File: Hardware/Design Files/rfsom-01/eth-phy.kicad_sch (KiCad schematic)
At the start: 50 parts, among them U6 KSZ9131RNXI-TR, Y3 ECS-2033-250-BN

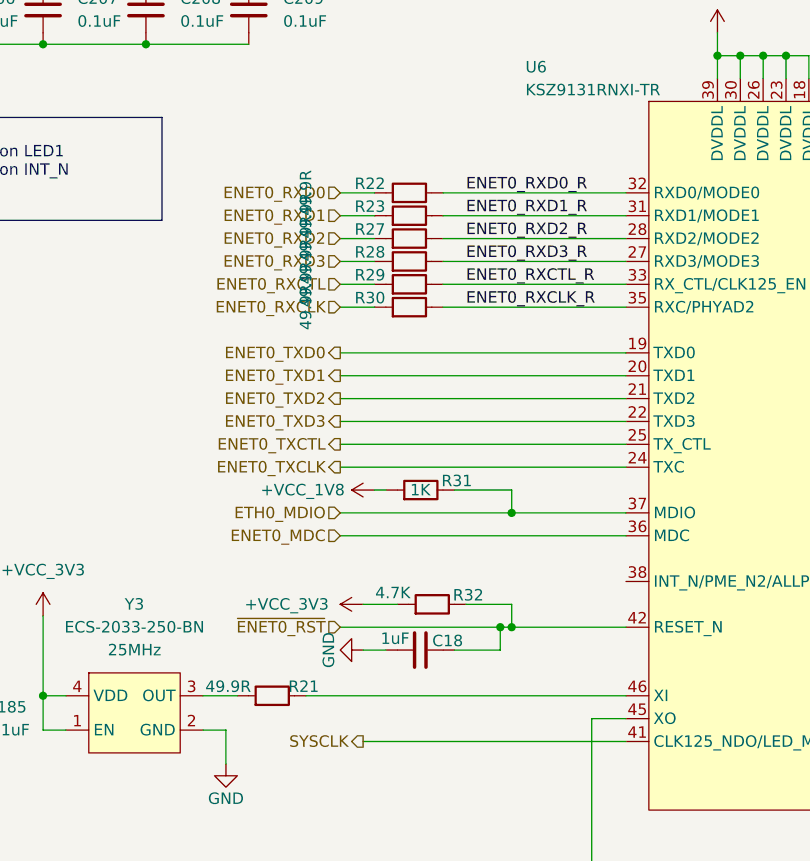
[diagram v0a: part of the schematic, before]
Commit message: updated sch pdf; routign progress;
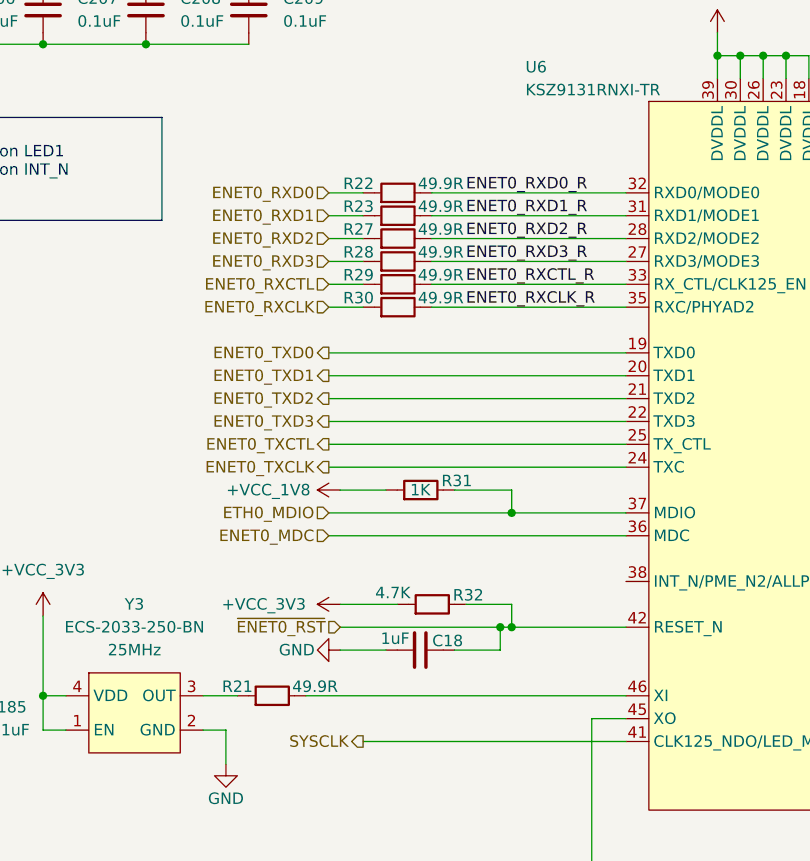
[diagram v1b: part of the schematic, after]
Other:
- moved on the sheet: R22, R23, R27, R28, R29, R30
